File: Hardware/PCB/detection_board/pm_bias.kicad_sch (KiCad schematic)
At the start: 0 parts

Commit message: Created detection board schematic
Created detection board schematic (AC)
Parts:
- added C1: 3 pF, Capacitor_SMD:C_0805_2012Metric, symbol Device:C
- added C2, C3: C, Package_DFN_QFN:QFN-20-1EP_4x4mm_P0.5mm_EP2.5x2.5mm, symbol Device:C
- added R1: 50 Ohms, Package_DIP:DIP-8_W7.62mm, symbol Device:R
- added R2, R4: R, Resistor_SMD:R_0805_2012Metric, symbol Device:R
- added R3: R, Package_DIP:DIP-8_W7.62mm, symbol Device:R
- added R5: 2.5 kOhm, Resistor_SMD:R_0805_2012Metric, symbol Device:R
- added R6: 50 Ohm, Resistor_SMD:R_0805_2012Metric, symbol Device:R
- added U1: MICROFC-60035-SMT-TR1, MICROFC-60035-SMT-TR1:XDCR_MICROFC-60035-SMT-TR1, symbol MICROFC-60035-SMT-TR1:MICROFC-60035-SMT-TR1
- added U2: ${SIM.PARAMS}, Package_TO_SOT_SMD:SOT-353_SC-70-5, symbol Simulation_SPICE:OPAMP
- added U3: LM397, Package_TO_SOT_SMD:SOT-23-5, symbol Comparator:LM397
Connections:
- new net: R5.2, R6.1, U3.1 (-)
- new net: C1.2, R1.1, R2.2, U2.5
- new net: R1.2, U3.3 (+)
- new net: C1.1, C3.2, R2.1, R4.2, U2.2 (-)
- new net: C2.2, R3.2, R4.1
- new net +5V: R5.1, U2.3 (V+), U3.5 (V+)
- new net -30V: R3.1, U1.1
- new net GND: C2.1, C3.1, R6.2, U1.3, U2.1 (+), U2.4 (V-), U3.2 (V-)

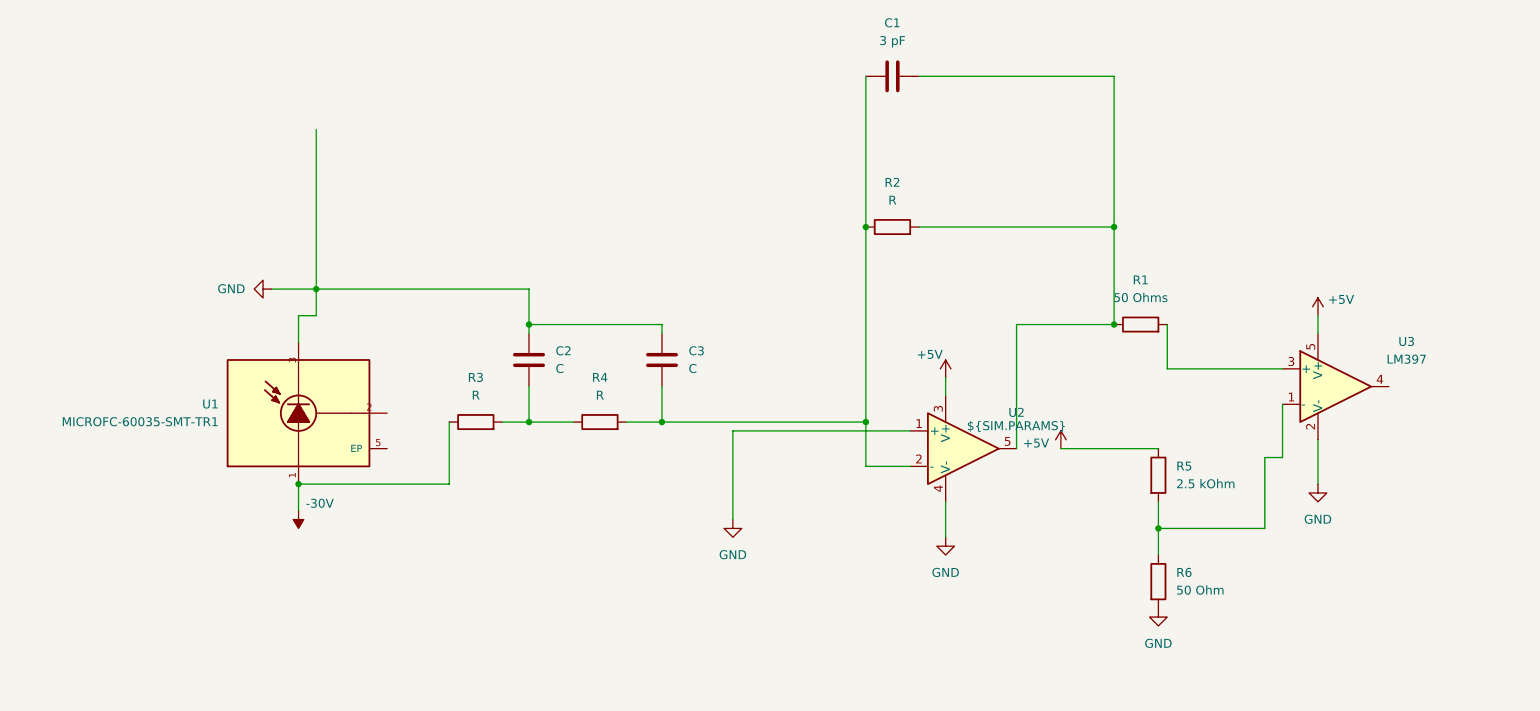
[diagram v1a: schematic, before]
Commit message: finished schem
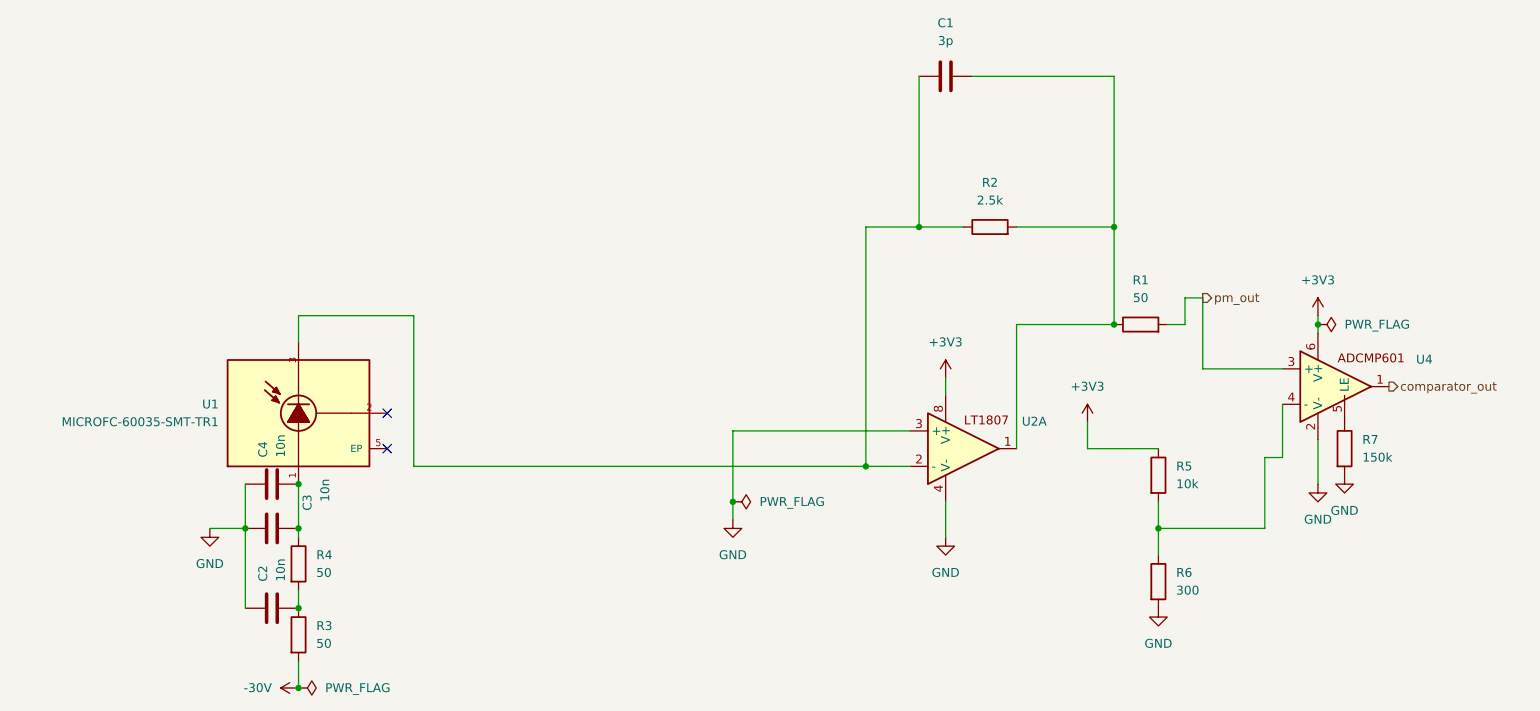
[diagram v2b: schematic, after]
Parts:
- removed U2: ${SIM.PARAMS}, Package_TO_SOT_SMD:SOT-353_SC-70-5, symbol Simulation_SPICE:OPAMP
- removed U3: LM397, Package_TO_SOT_SMD:SOT-23-5, symbol Comparator:LM397
- added C4: 10n, Capacitor_SMD:C_0805_2012Metric, symbol Device:C
- added R7: 150k, Resistor_SMD:R_0805_2012Metric, symbol Device:R
- added U2: (no value), Package_SO:SOIC-8_3.9x4.9mm_P1.27mm, symbol New_Library:LT1807
- added U4: (no value), Package_TO_SOT_SMD:SOT-363_SC-70-6, symbol New_Library:ADCMP601
- C1: value 3 pF -> 3p
- C2, C3: value C -> 10n; footprint Package_DFN_QFN:QFN-20-1EP_4x4mm_P0.5mm_EP2.5x2.5mm -> Capacitor_SMD:C_0805_2012Metric
- R1: value 50 Ohms -> 50; footprint Package_DIP:DIP-8_W7.62mm -> Resistor_SMD:R_0805_2012Metric
- R2: value R -> 2.5k
- R3: value R -> 50; footprint Package_DIP:DIP-8_W7.62mm -> Resistor_SMD:R_0805_2012Metric
- R4: value R -> 50
- R5: value 2.5 kOhm -> 10k
- R6: value 50 Ohm -> 300
- U1: footprint MICROFC-60035-SMT-TR1:XDCR_MICROFC-60035-SMT-TR1 -> micro:XDCR_MICROFC-60035-SMT-TR1
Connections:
- net -30V: now also R3.2; no longer R3.1, U1.1
- net GND: now also C4.1, R7.2, U2.3 (+), U2.4 (V-), U4.2 (V-); no longer U1.3
- net at R5.2, R6.1: now also U4.4 (-)
- net at C1.2, R1.1, R2.2: now also U2.1
- net pm_out: now reaches R1.2
- net pm_out: now also U4.3 (+)
- net at C1.1, R2.1: now also U1.3, U2.2 (-); no longer C3.2, R4.2
- net +5V renamed +3V3
- net +3V3: now also U2.8 (V+), U4.6 (V+)
- new net: R7.1, U4.5 (LE)
- new net: C2.2, R3.1, R4.2
- new net: C3.2, C4.2, R4.1, U1.1
- new net comparator_out: U4.1
- no-connect marks 0 -> 2
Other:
- moved on the sheet: C1, R2
